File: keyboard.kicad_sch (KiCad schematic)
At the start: 24 parts, among them SW1 RESET, U1 ATmega32U4-A, Y1 16MHz

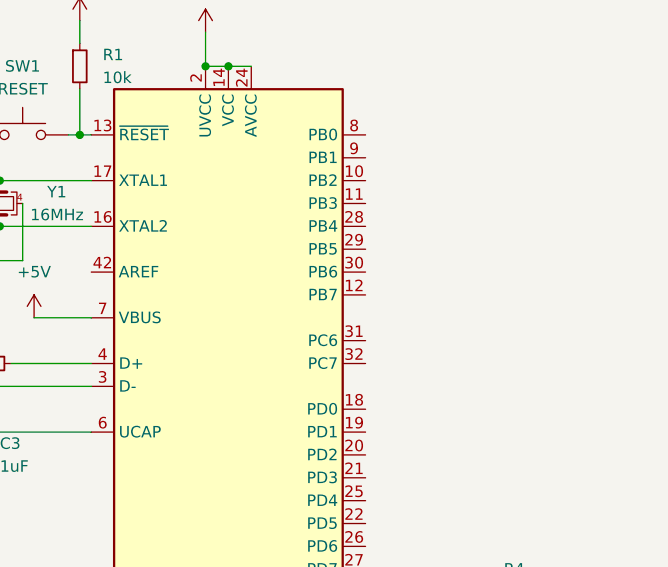
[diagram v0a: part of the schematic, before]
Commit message: PCB done
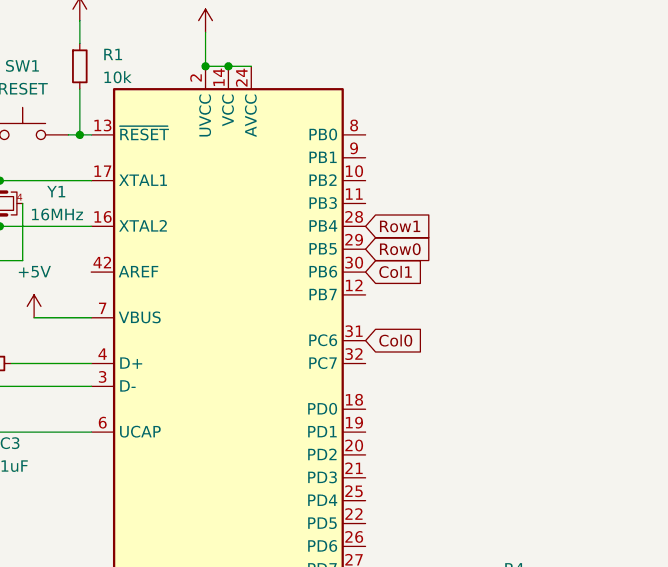
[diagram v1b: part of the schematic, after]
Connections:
- net Col0: now also U1.31 (PC6)
- net Col1: now also U1.30 (PB6)
- net Row0: now also U1.29 (PB5)
- net Row1: now also U1.28 (PB4)
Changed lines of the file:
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@@
     (stroke (width 0) (type default))
+  )
+  (global_label "Row1" (shape input) (at 250.19 44.45 0) (fields_autoplaced)
+    (effects (font (size 1.27 1.27)) (justify left))
+    (property "Intersheetrefs" "${INTERSHEET_REFS}" (at 258.1342 44.45 0)
+      (effects (font (size 1.27 1.27)) (justify left) hide)
+    )
   )
   (global_label "Col1" (shape input) (at 182.88 123.19 90) (fields_autoplaced)
@@
     )
   )
+  (global_label "Row0" (shape input) (at 250.19 46.99 0) (fields_autoplaced)
+    (effects (font (size 1.27 1.27)) (justify left))
+    (property "Intersheetrefs" "${INTERSHEET_REFS}" (at 258.1342 46.99 0)
+      (effects (font (size 1.27 1.27)) (justify left) hide)
+    )
+  )
   (global_label "D-" (shape input) (at 193.04 62.23 180) (fields_autoplaced)
     (effects (font (size 1.27 1.27)) (justify right))
@@
     )
   )
+  (global_label "Col1" (shape input) (at 250.19 49.53 0) (fields_autoplaced)
+    (effects (font (size 1.27 1.27)) (justify left))
+    (property "Intersheetrefs" "${INTERSHEET_REFS}" (at 257.4689 49.53 0)
+      (effects (font (size 1.27 1.27)) (justify left) hide)
+    )
+  )
   (global_label "Row1" (shape input) (at 153.67 158.75 180) (fields_autoplaced)
     (effects (font (size 1.27 1.27)) (justify right))
@@
     )
   )
+  (global_label "Col0" (shape input) (at 250.19 57.15 0) (fields_autoplaced)
+    (effects (font (size 1.27 1.27)) (justify left))
+    (property "Intersheetrefs" "${INTERSHEET_REFS}" (at 257.4689 57.15 0)
+      (effects (font (size 1.27 1.27)) (justify left) hide)
+    )
+  )
